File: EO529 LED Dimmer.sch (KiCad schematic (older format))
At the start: 47 parts, among them J1 VBat, Q1 BC639, Q2 BC639, Q3 BC639, Q4 BC639, U1 NE556, U2 NE556

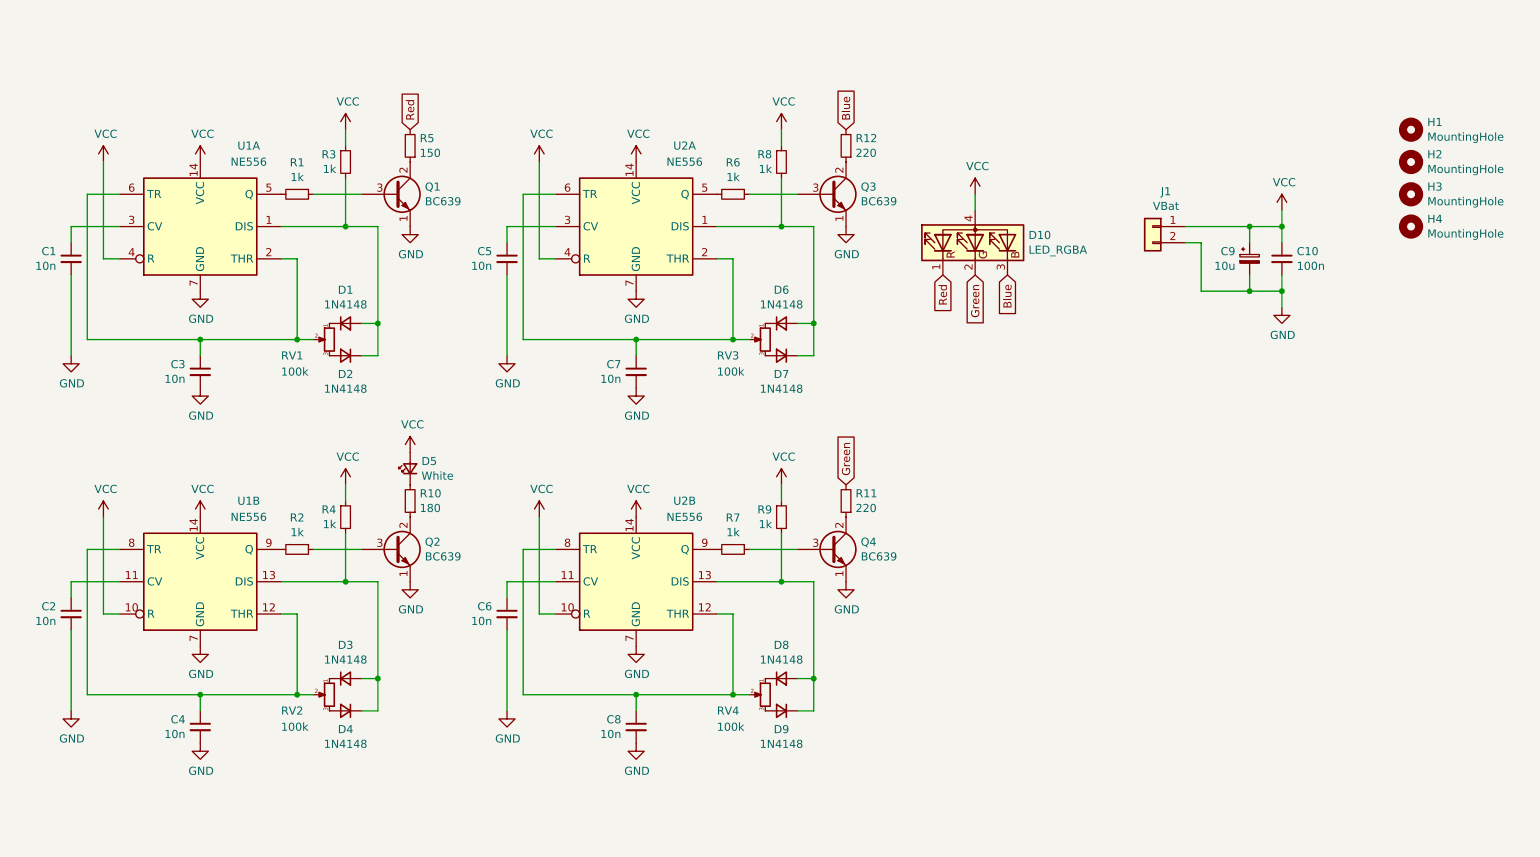
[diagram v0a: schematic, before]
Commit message: Revision to circuit
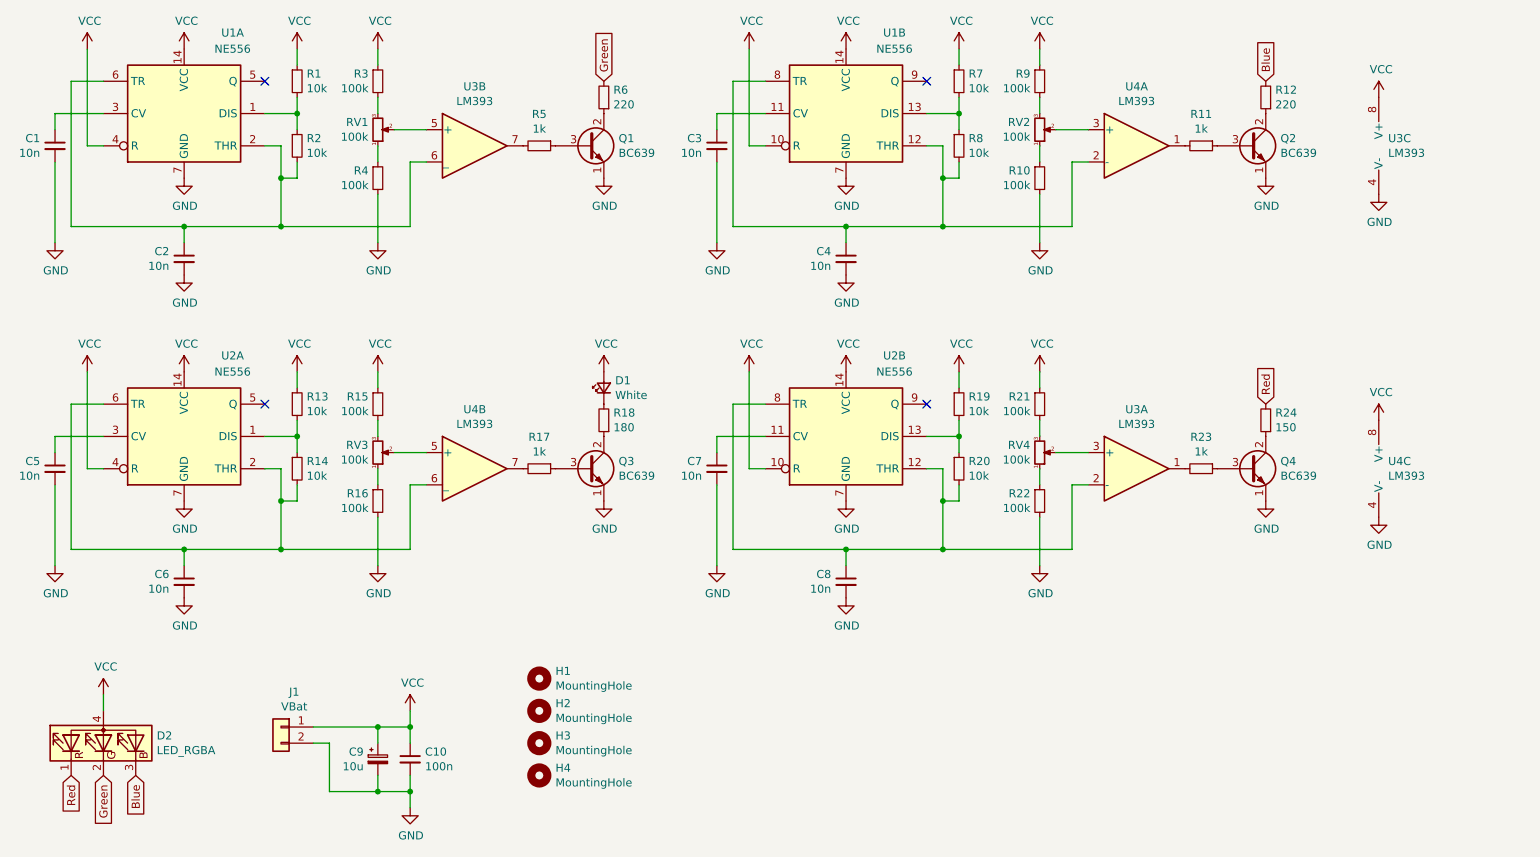
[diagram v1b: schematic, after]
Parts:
- removed C2: 10n, Capacitor_THT:C_Disc_D5.0mm_W2.5mm_P5.00mm, symbol Device:C_Small
- removed D1, D2, D3, D4, D6, D7, D8, D9: 1N4148, Diode_THT:D_DO-35_SOD27_P7.62mm_Horizontal, symbol Device:D_Small
- removed D10: LED_RGBA, LED_THT:LED_BL-FL7680RGB, symbol Device:LED_RGBA
- removed D5: White, LED_THT:LED_D10.0mm, symbol Device:LED_Small
- removed R6: 1k, Resistor_THT:R_Axial_DIN0207_L6.3mm_D2.5mm_P7.62mm_Horizontal, symbol Device:R_Small
- added C3: 10n, Capacitor_THT:C_Disc_D5.0mm_W2.5mm_P5.00mm, symbol Device:C_Small
- added D1: White, LED_THT:LED_D10.0mm, symbol Device:LED_Small
- added D2: LED_RGBA, LED_THT:LED_BL-FL7680RGB, symbol Device:LED_RGBA
- added R13, R14, R19, R20: 10k, Resistor_THT:R_Axial_DIN0207_L6.3mm_D2.5mm_P7.62mm_Horizontal, symbol Device:R_Small
- added R15, R16, R21, R22, R3: 100k, Resistor_THT:R_Axial_DIN0207_L6.3mm_D2.5mm_P7.62mm_Horizontal, symbol Device:R_Small
- added R17, R23: 1k, Resistor_THT:R_Axial_DIN0207_L6.3mm_D2.5mm_P7.62mm_Horizontal, symbol Device:R_Small
- added R18: 180, Resistor_THT:R_Axial_DIN0207_L6.3mm_D2.5mm_P7.62mm_Horizontal, symbol Device:R_Small
- added R24: 150, Resistor_THT:R_Axial_DIN0207_L6.3mm_D2.5mm_P7.62mm_Horizontal, symbol Device:R_Small
- added U3, U4: LM393, Package_DIP:DIP-8_W7.62mm_Socket, symbol Comparator:LM393
- R1: renamed from R3; value 1k -> 10k
- R10: value 180 -> 100k
- R11: value 220 -> 1k
- R2, R7, R8: value 1k -> 10k
- R4, R9: value 1k -> 100k
- R6: renamed from R5; value 150 -> 220
- renumbered C3 to C2, R1 to R5
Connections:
- net Blue: now also D2.3 (BK)
- net GND: now also R10.2, R4.2, C3.2, R16.2, R22.2, U3.4 (V-), U4.4 (V-)
- net Green: now also R6.2, D2.2 (GK); no longer R11.2
- net Red: now also D2.1 (RK), R24.2; no longer R6.2
- net VCC: now also R7.1, D1.2 (A), D2.4 (A), R13.1, R15.1, R19.1, R21.1, R3.1, U3.8 (V+), U4.8 (V+); no longer R4.1, R8.1
- net at R1.2, U1.1 (DIS): now also R2.1
- net at C2.1, U1.2 (THR), U1.6 (TR): now also R2.2, U3.6 (_); no longer RV1.2
- net at U1.5 (Q): no longer R5.2
- net at R8.2: now also C4.1, U1.12 (THR), U1.8 (TR), U4.2 (-); no longer U2.1 (DIS)
- net at U2.2 (THR), U2.6 (TR): now also C6.1, R14.2, U4.6 (_); no longer C7.1, RV3.2
- net at RV1.1: now also R4.1
- net at RV1.3: now also R3.2
- net at RV3.1: now also R16.1
- net at Q3.3 (B): now also R17.1
- net at R11.1: now also Q2.3 (B); no longer Q4.2 (C)
- net at RV3.3: now also R15.2
- net at R12.1: now also Q2.2 (C); no longer Q3.2 (C)
- net at U1.11 (CV): now also C3.1
- net at U1.13 (DIS): now also R7.2, R8.1; no longer R4.2
- net at U1.9 (Q): no longer R2.2
- net at U2.11 (CV): now also C7.1; no longer C6.1
- net at C8.1, U2.12 (THR), U2.8 (TR): now also R20.2, U3.2 (-); no longer RV4.2
- net at R9.2: now also RV2.3; no longer U2.13 (DIS)
- net at U2.9 (Q): no longer R7.2
- net at RV2.1: now also R10.1
- net at RV4.1: now also R22.1
- net at Q4.3 (B): now also R23.1; no longer R7.1
- net at RV4.3: now also R21.2
- new net: RV1.2, U3.5 (+)
- new net: R5.2, U3.7
- new net: R11.2, U4.1
- new net: RV2.2, U4.3 (+)
- new net: RV3.2, U4.5 (+)
- new net: R17.2, U4.7
- new net: R13.2, R14.1, U2.1 (DIS)
- new net: Q3.2 (C), R18.1
- new net: D1.1 (K), R18.2
- new net: R19.2, R20.1, U2.13 (DIS)
- new net: R23.2, U3.1
- new net: RV4.2, U3.3 (+)
- new net: Q4.2 (C), R24.1
- no-connect marks 0 -> 4
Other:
- moved on the sheet: C1, C10, C2, C9, H1, H2, H3, H4, J1, Q1, R1, R5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
